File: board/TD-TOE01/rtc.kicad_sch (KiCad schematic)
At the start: 4 parts, among them U11 DS1307, Y2 32.768KHz

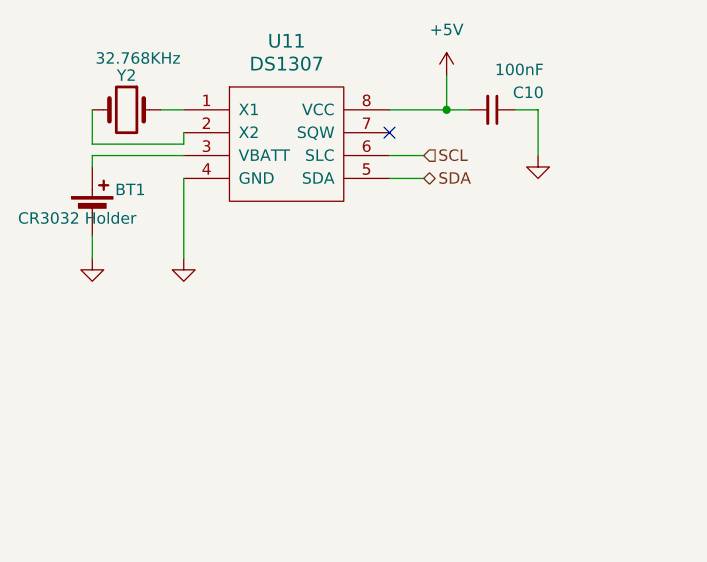
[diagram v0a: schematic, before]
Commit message: OET PCB
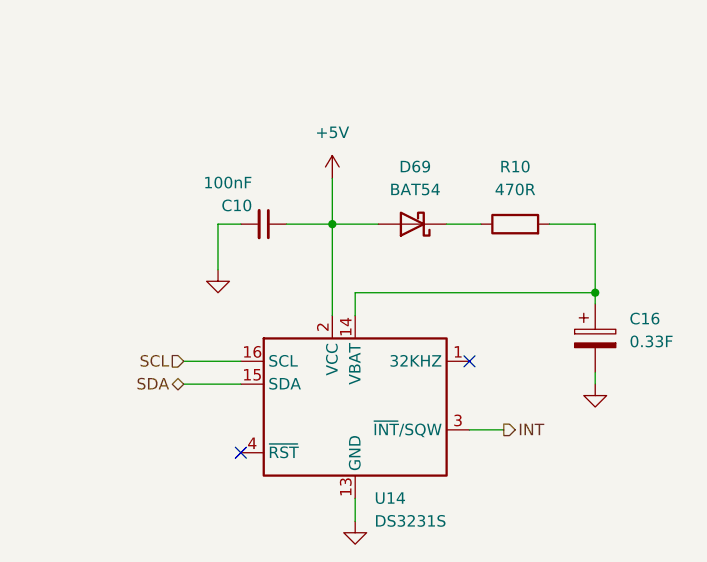
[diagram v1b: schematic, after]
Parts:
- removed BT1: CR3032 Holder, TokeiDigital:CR2032 Holder, symbol TokeiDigital:Battery_Cell
- removed U11: DS1307, TokeiDigital:SOIC-8, symbol TokeiDigital:DS1307
- removed Y2: 32.768KHz, TokeiDigital:Crystal Horizontal, symbol TokeiDigital:Crystal
- added C16: 0.33F, TokeiDigital:StarcapSuperCap-HType, symbol TokeiDigital:C_Polarized
- added D69: BAT54, Package_TO_SOT_SMD:TSOT-23, symbol TokeiDigital:BAT54
- added R10: 470R, TokeiDigital:R_0805, symbol Device:R
- added U14: DS3231S, Package_SO:SOIC-16W_7.5x10.3mm_P1.27mm, symbol TokeiDigital:DS3231M
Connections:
- net +5V: now also C10.1, D69.1 (A), U14.2 (VCC); no longer C10.2
- net GND: now also C10.2, C16.2, U14.10 (GND), U14.11 (GND), U14.12 (GND), U14.13 (GND), U14.5 (GND), U14.6 (GND), U14.7 (GND), U14.8 (GND), U14.9 (GND); no longer C10.1
- net SCL: now also U14.16 (SCL)
- net SDA: now also U14.15 (SDA)
- new net: D69.3 (K), R10.1
- new net: C16.1, R10.2, U14.14 (VBAT)
- new net INT: U14.3 (~{INT}/SQW)
- no-connect marks 1 -> 2
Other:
- moved on the sheet: C10
